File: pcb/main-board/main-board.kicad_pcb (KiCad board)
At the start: 2 copper layers, 97.3 x 40.6 mm, 27 parts, among them J1 Conn_01x07, J2 Conn_01x05, P1 USB_C_Plug_USB2.0, SW1 SW_Push, SW2 RESET, SW3 PROG, U1 ESP32-WROOM-32, U2 PC817, U3 PC817, U4 PC817, U5 PC817, U6 AMS1117

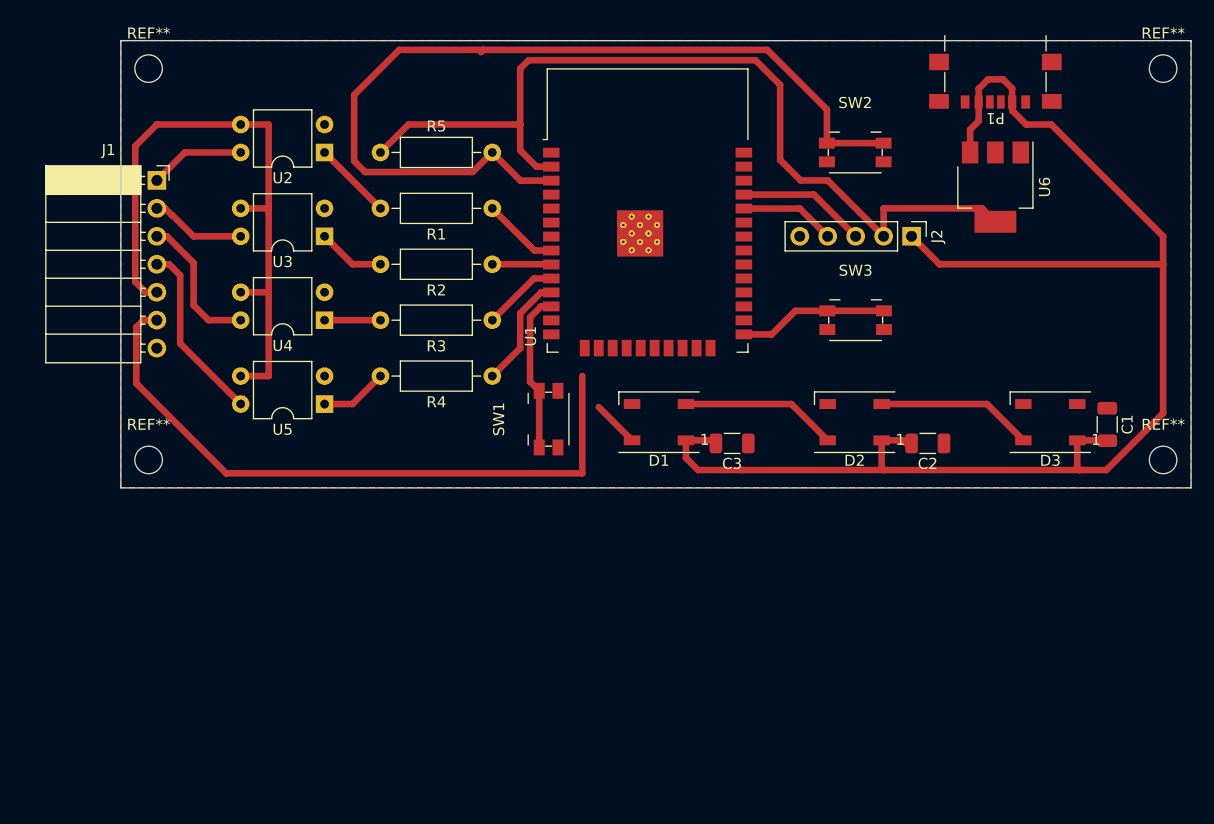
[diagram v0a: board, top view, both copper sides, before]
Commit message: New PCB & case
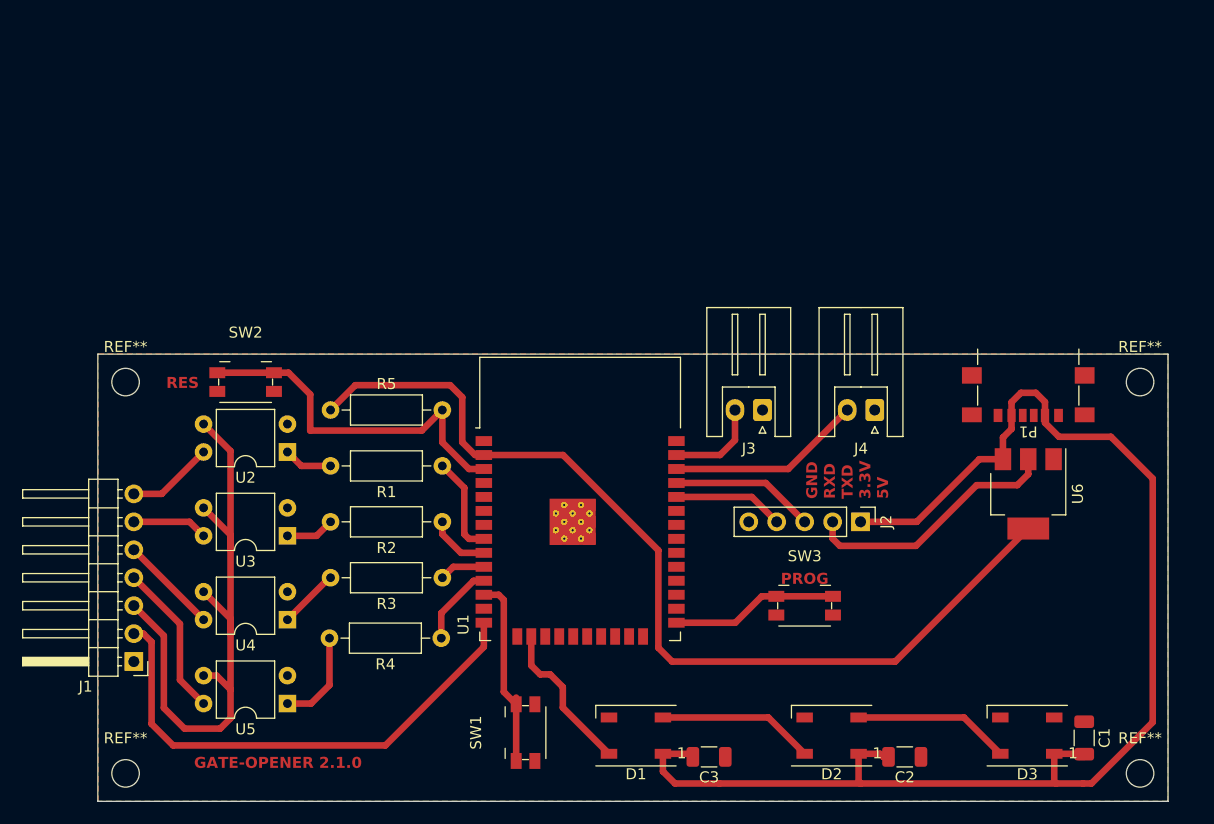
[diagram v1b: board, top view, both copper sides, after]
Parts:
- added J3: Conn_01x02, Connector_JST:JST_XH_S2B-XH-A_1x02_P2.50mm_Horizontal, F.Cu at (177.0, 84.4)
- added J4: Conn_01x02, Connector_JST:JST_XH_S2B-XH-A_1x02_P2.50mm_Horizontal, F.Cu at (187.2, 84.4)
- J1: footprint Connector_PinSocket_2.54mm:PinSocket_1x07_P2.54mm_Horizontal -> Connector_PinHeader_2.54mm:PinHeader_1x07_P2.54mm_Horizontal
- REF**: value MountingHole_2.2mm_M2 -> locked
- moved SW2 59.2 mm to (130.0, 81.8)
- moved J1 43.8 mm to (119.8, 107.2), turned to 180 degrees
- moved P1 28.6 mm to (201.1, 81.8)
- moved SW1 28.6 mm to (155.4, 113.7)
- moved C1 28.6 mm to (206.2, 114.2)
- moved C2 28.6 mm to (189.9, 115.9)
- moved C3 28.6 mm to (172.1, 115.9)
- moved D1 28.6 mm to (165.5, 114.0)
- moved D2 28.6 mm to (183.2, 114.0)
- moved D3 28.6 mm to (201.0, 114.0)
- moved REF** 28.6 mm to (211.3, 117.4)
- moved REF** 28.6 mm to (119.1, 117.4)
- moved REF** 28.6 mm to (211.3, 81.8)
- moved REF** 28.6 mm to (119.1, 81.8)
- moved U6 28.0 mm to (201.1, 92.0)
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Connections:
- J1 pad 1: RE1 -> GND
- J1 pad 2: RE2 -> IO12
- J1 pad 3: RE3 -> GND2
- J1 pad 5: GND2 -> RE3
- J1 pad 6: IO12 -> RE2
- J1 pad 7: GND -> RE1
- U1 pad 36: unconnected-(U1-IO22-Pad36) -> IO22
- U1 pad 37: unconnected-(U1-IO23-Pad37) -> IO23
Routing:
- net EN: track 81.5 -> 33.0 mm
- net 3.3V: track 81.8 -> 111.0 mm
- net IO22: track 0.00 -> 17.7 mm
- net IO12: track 60.0 -> 46.3 mm
- net IO13: track 4.28 -> 14.1 mm
- net IO23: track 0.00 -> 8.62 mm
- net 5V: track 131.9 -> 123.4 mm
- net RE3: track 13.0 -> 8.98 mm
- net IO27: track 14.5 -> 17.7 mm
- net IO26: track 10.4 -> 7.36 mm
- net IO25: track 6.93 -> 4.18 mm
- net Net-(R1-Pad2): track 7.18 -> 4.44 mm
- net Net-(R4-Pad2): track 6.13 -> 8.78 mm
- net RE4: track 16.5 -> 14.1 mm
- net IO32: track 6.95 -> 8.98 mm
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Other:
- board text added: "GATE-OPENER 2.1.0"
- board text added: "GND RXD TXD 3.3V 5V"
- board text added: "PROG"
- board text added: "RES"
